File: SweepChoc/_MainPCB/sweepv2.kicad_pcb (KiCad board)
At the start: 2 copper layers, 216.9 x 86.9 mm, 59 parts, among them J1 AudioJack4dpb, J2 AudioJack4dpb, SW1 SW_Push, SW10 SW_Push, SW11 SW_Push, SW11_r1 SW_Push, SW12 SW_Push, SW12_r1 SW_Push, SW13_r1 SW_Push, SW14 SW_Push, SW15 SW_Push, SW15_r1 SW_Push, SW16 SW_Push, SW16_r1 SW_Push, SW17 SW_Push, SW17_r1 SW_Push, SW18 SW_Push, SW18_r1 SW_Push, SW2 SW_Push, SW20 SW_Push, SW21 SW_Push, SW2_r1 SW_Push, SW3 SW_Push, SW3_r1 SW_Push, SW4 SW_Push, SW4_r1 SW_Push, SW5 SW_Push, SW5_r1 SW_Push, SW6 SW_Push, SW6_r1 SW_Push, SW7 SW_Push, SW7_r1 SW_Push, SW8 SW_Push, SW8_r1 SW_Push, SW9 SW_Push, SW9_r1 SW_Push, U1 ProMicro-kbd, U2 ProMicro-kbd

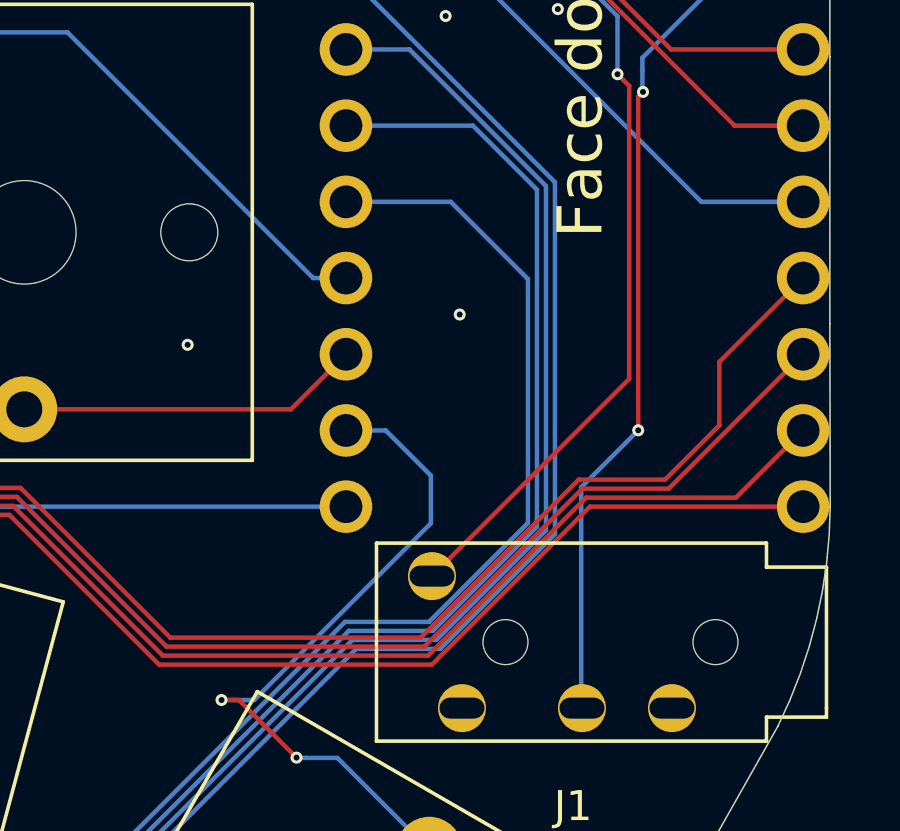
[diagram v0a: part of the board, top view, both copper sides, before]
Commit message: rename of some bits and a couple missed fixes
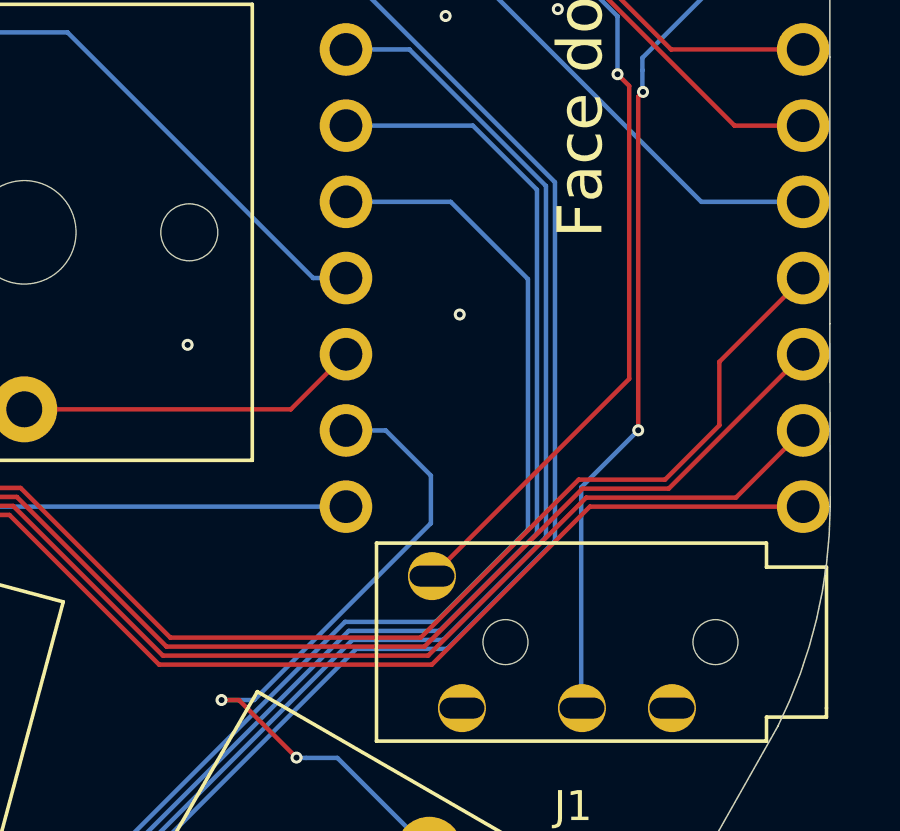
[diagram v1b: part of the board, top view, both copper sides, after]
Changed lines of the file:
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@@
   (segment (start 218.425 59.4) (end 218.425 57.727) (width 0.15) (layer "B.Cu") (net 14))
   (segment (start 218.425 57.727) (end 222.558 53.594) (width 0.15) (layer "B.Cu") (net 14))
-  (segment (start 229.525 82.45) (end 229.525 70.721) (width 0.15) (layer "B.Cu") (net 15))
+  (segment (start 144.893 89.282) (end 149.6 84.575) (width 0.15) (layer "B.Cu") (net 15))
+  (segment (start 225.925 86.275) (end 229.525 82.675) (width 0.15) (layer "B.Cu") (net 15))
+  (segment (start 214.425 94.75) (end 222.9 86.275) (width 0.15) (layer "B.Cu") (net 15))
+  (segment (start 222.9 86.275) (end 225.925 86.275) (width 0.15) (layer "B.Cu") (net 15))
+  (segment (start 229.525 82.675) (end 229.525 70.721) (width 0.15) (layer "B.Cu") (net 15))
+  (segment (start 229.525 70.721) (end 222.558 63.754) (width 0.15) (layer "B.Cu") (net 15))
+  (segment (start 149.6 84.575) (end 188.3 84.575) (width 0.15) (layer "B.Cu") (net 15))
+  (segment (start 198.475 94.75) (end 214.425 94.75) (width 0.15) (layer "B.Cu") (net 15))
+  (segment (start 188.3 84.575) (end 198.475 94.75) (width 0.15) (layer "B.Cu") (net 15))
   (segment (start 139.856 89.282) (end 144.893 89.282) (width 0.15) (layer "B.Cu") (net 15))
-  (segment (start 229.525 70.721) (end 222.558 63.754) (width 0.15) (layer "B.Cu") (net 15))
-  (segment (start 188.3 84.575) (end 198.475 94.75) (width 0.15) (layer "B.Cu") (net 15))
-  (segment (start 214.425 94.75) (end 222.9 86.275) (width 0.15) (layer "B.Cu") (net 15))
-  (segment (start 149.6 84.575) (end 188.3 84.575) (width 0.15) (layer "B.Cu") (net 15))
-  (segment (start 222.9 86.275) (end 225.7 86.275) (width 0.15) (layer "B.Cu") (net 15))
-  (segment (start 144.893 89.282) (end 149.6 84.575) (width 0.15) (layer "B.Cu") (net 15))
-  (segment (start 198.475 94.75) (end 214.425 94.75) (width 0.15) (layer "B.Cu") (net 15))
-  (segment (start 225.7 86.275) (end 229.525 82.45) (width 0.15) (layer "B.Cu") (net 15))
-  (segment (start 229.225 70.845264) (end 229.225 82.325736) (width 0.15) (layer "B.Cu") (net 16))
-  (segment (start 225.575736 85.975) (end 222.775736 85.975) (width 0.15) (layer "B.Cu") (net 16))
+  (segment (start 225.800736 85.975) (end 222.775736 85.975) (width 0.15) (layer "B.Cu") (net 16))
+  (segment (start 214.300736 94.45) (end 198.599264 94.45) (width 0.15) (layer "B.Cu") (net 16))
+  (segment (start 222.558 66.294) (end 224.673736 66.294) (width 0.15) (layer "B.Cu") (net 16))
+  (segment (start 164.475 84.275) (end 157.856 77.656) (width 0.15) (layer "B.Cu") (net 16))
+  (segment (start 157.856 77.656) (end 157.856 77.274) (width 0.15) (layer "B.Cu") (net 16))
+  (segment (start 188.424264 84.275) (end 164.475 84.275) (width 0.15) (layer "B.Cu") (net 16))
   (segment (start 198.599264 94.45) (end 188.424264 84.275) (width 0.15) (layer "B.Cu") (net 16))
-  (segment (start 222.558 66.294) (end 224.673736 66.294) (width 0.15) (layer "B.Cu") (net 16))
-  (segment (start 188.424264 84.275) (end 164.475 84.275) (width 0.15) (layer "B.Cu") (net 16))
-  (segment (start 229.225 82.325736) (end 225.575736 85.975) (width 0.15) (layer "B.Cu") (net 16))
   (segment (start 222.775736 85.975) (end 214.300736 94.45) (width 0.15) (layer "B.Cu") (net 16))
-  (segment (start 164.475 84.275) (end 157.856 77.656) (width 0.15) (layer "B.Cu") (net 16))
   (segment (start 224.673736 66.294) (end 229.225 70.845264) (width 0.15) (layer "B.Cu") (net 16))
-  (segment (start 157.856 77.656) (end 157.856 77.274) (width 0.15) (layer "B.Cu") (net 16))
-  (segment (start 214.300736 94.45) (end 198.599264 94.45) (width 0.15) (layer "B.Cu") (net 16))
+  (segment (start 229.225 82.550736) (end 225.800736 85.975) (width 0.15) (layer "B.Cu") (net 16))
+  (segment (start 229.225 70.845264) (end 229.225 82.550736) (width 0.15) (layer "B.Cu") (net 16))
+  (segment (start 214.176472 94.15) (end 198.723528 94.15) (width 0.15) (layer "B.Cu") (net 17))
+  (segment (start 225.676472 85.675) (end 222.651472 85.675) (width 0.15) (layer "B.Cu") (net 17))
+  (segment (start 228.925 82.426472) (end 225.676472 85.675) (width 0.15) (layer "B.Cu") (net 17))
+  (segment (start 175.856 78.906) (end 175.856 70.416) (width 0.15) (layer "B.Cu") (net 17))
+  (segment (start 228.925 70.969528) (end 228.925 82.426472) (width 0.15) (layer "B.Cu") (net 17))
+  (segment (start 222.558 68.834) (end 226.789472 68.834) (width 0.15) (layer "B.Cu") (net 17))
+  (segment (start 188.548528 83.975) (end 180.925 83.975) (width 0.15) (layer "B.Cu") (net 17))
+  (segment (start 180.925 83.975) (end 175.856 78.906) (width 0.15) (layer "B.Cu") (net 17))
+  (segment (start 198.723528 94.15) (end 188.548528 83.975) (width 0.15) (layer "B.Cu") (net 17))
   (segment (start 226.789472 68.834) (end 228.925 70.969528) (width 0.15) (layer "B.Cu") (net 17))
-  (segment (start 214.176472 94.15) (end 198.723528 94.15) (width 0.15) (layer "B.Cu") (net 17))
-  (segment (start 228.925 82.201472) (end 225.451472 85.675) (width 0.15) (layer "B.Cu") (net 17))
-  (segment (start 188.548528 83.975) (end 180.925 83.975) (width 0.15) (layer "B.Cu") (net 17))
-  (segment (start 228.925 70.969528) (end 228.925 82.201472) (width 0.15) (layer "B.Cu") (net 17))
-  (segment (start 222.558 68.834) (end 226.789472 68.834) (width 0.15) (layer "B.Cu") (net 17))
   (segment (start 222.651472 85.675) (end 214.176472 94.15) (width 0.15) (layer "B.Cu") (net 17))
-  (segment (start 198.723528 94.15) (end 188.548528 83.975) (width 0.15) (layer "B.Cu") (net 17))
-  (segment (start 225.451472 85.675) (end 222.651472 85.675) (width 0.15) (layer "B.Cu") (net 17))
-  (segment (start 175.856 78.906) (end 175.856 70.416) (width 0.15) (layer "B.Cu") (net 17))
-  (segment (start 180.925 83.975) (end 175.856 78.906) (width 0.15) (layer "B.Cu") (net 17))
+  (segment (start 226.049 71.374) (end 228.625 73.95) (width 0.15) (layer "B.Cu") (net 18))
   (segment (start 193.856 88.858208) (end 193.856 75.75) (width 0.15) (layer "B.Cu") (net 18))
-  (segment (start 225.327208 85.375) (end 222.527208 85.375) (width 0.15) (layer "B.Cu") (net 18))
+  (segment (start 225.552208 85.375) (end 222.527208 85.375) (width 0.15) (layer "B.Cu") (net 18))
+  (segment (start 222.558 71.374) (end 226.049 71.374) (width 0.15) (layer "B.Cu") (net 18))
+  (segment (start 198.847792 93.85) (end 193.856 88.858208) (width 0.15) (layer "B.Cu") (net 18))
+  (segment (start 222.527208 85.375) (end 214.052208 93.85) (width 0.15) (layer "B.Cu") (net 18))
+  (segment (start 228.625 73.95) (end 228.625 82.302208) (width 0.15) (layer "B.Cu") (net 18))
   (segment (start 214.052208 93.85) (end 198.847792 93.85) (width 0.15) (layer "B.Cu") (net 18))
-  (segment (start 226.049 71.374) (end 228.625 73.95) (width 0.15) (layer "B.Cu") (net 18))
-  (segment (start 222.558 71.374) (end 226.049 71.374) (width 0.15) (layer "B.Cu") (net 18))
-  (segment (start 222.527208 85.375) (end 214.052208 93.85) (width 0.15) (layer "B.Cu") (net 18))
-  (segment (start 198.847792 93.85) (end 193.856 88.858208) (width 0.15) (layer "B.Cu") (net 18))
-  (segment (start 228.625 73.95) (end 228.625 82.077208) (width 0.15) (layer "B.Cu") (net 18))
-  (segment (start 228.625 82.077208) (end 225.327208 85.375) (width 0.15) (layer "B.Cu") (net 18))
+  (segment (start 228.625 82.302208) (end 225.552208 85.375) (width 0.15) (layer "B.Cu") (net 18))
   (segment (start 220.722 78.29) (end 211.836 78.29) (width 0.15) (layer "F.Cu") (net 19))
   (segment (start 222.558 76.454) (end 220.722 78.29) (width 0.15) (layer "F.Cu") (net 19))
